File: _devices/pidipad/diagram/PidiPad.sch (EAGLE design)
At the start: 25 parts, among them IC1 CH32V006E8R6, IC2 HT7533-1, K2 MICROSD, Q1 25 MHz, X1 USB, X2 VGA, X3 AUDIO, X4 SWIO

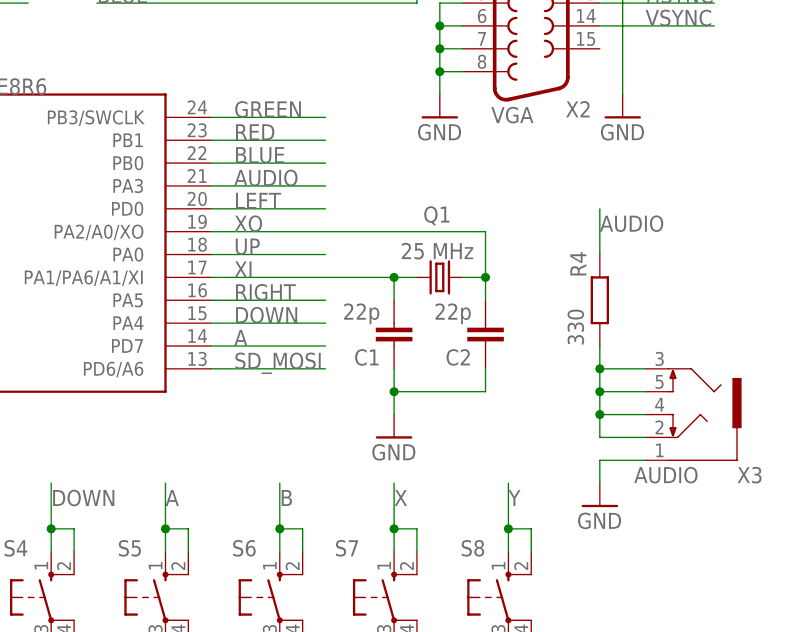
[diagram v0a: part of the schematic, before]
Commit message: init
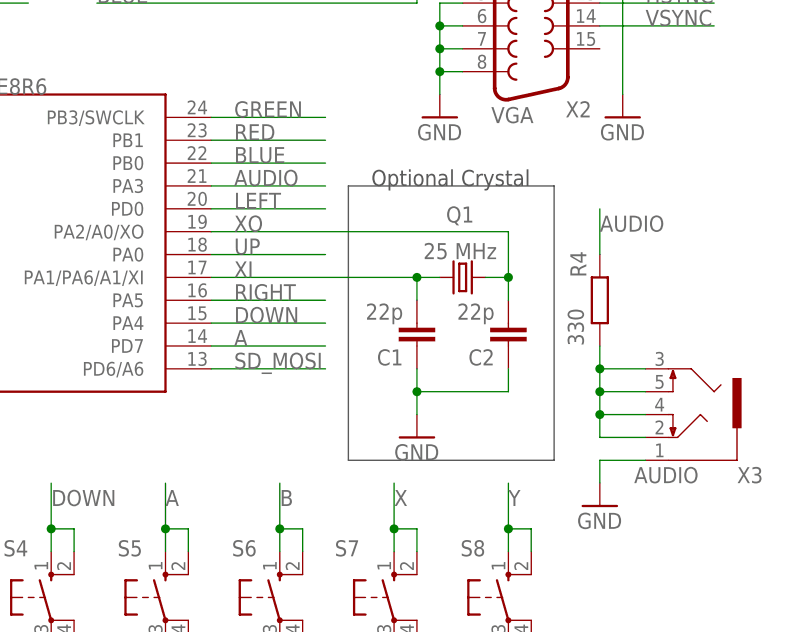
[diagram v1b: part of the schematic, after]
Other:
- note added: "Optional Crystal"
- moved on the sheet: C1, C2, Q1
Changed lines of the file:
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@@
 <setting verticaltext="up"/>
 </settings>
-<grid distance="100" unitdist="mil" unit="mil" style="lines" multiple="1" display="no" altdistance="0.01" altunitdist="inch" altunit="inch"/>
+<grid distance="0.1" unitdist="inch" unit="inch" style="lines" multiple="1" display="no" altdistance="0.01" altunitdist="inch" altunit="inch"/>
 <layers>
 <layer number="1" name="Top" color="4" fill="1" visible="no" active="no"/>
@@
 <text x="-86.36" y="0" size="1.778" layer="91">GND</text>
 <text x="-86.36" y="-2.54" size="1.778" layer="91">SWIO</text>
+<wire x1="17.78" y1="-27.94" x2="40.64" y2="-27.94" width="0.1524" layer="97"/>
+<wire x1="40.64" y1="-27.94" x2="40.64" y2="2.54" width="0.1524" layer="97"/>
+<wire x1="40.64" y1="2.54" x2="17.78" y2="2.54" width="0.1524" layer="97"/>
+<wire x1="17.78" y1="2.54" x2="17.78" y2="-27.94" width="0.1524" layer="97"/>
+<text x="20.32" y="2.54" size="1.778" layer="97">Optional Crystal</text>
 </plain>
 <instances>
@@
 <attribute name="VALUE" x="-33.02" y="12.7" size="1.778" layer="96"/>
 </instance>
-<instance part="Q1" gate="G$1" x="27.94" y="-7.62" rot="R180">
-<attribute name="NAME" x="29.21" y="0.254" size="1.778" layer="95" rot="R180"/>
-<attribute name="VALUE" x="31.75" y="-3.81" size="1.778" layer="96" rot="R180"/>
-</instance>
-<instance part="C1" gate="G$1" x="22.86" y="-15.24" rot="R180">
-<attribute name="NAME" x="21.336" y="-15.621" size="1.778" layer="95" rot="R180"/>
-<attribute name="VALUE" x="21.336" y="-10.541" size="1.778" layer="96" rot="R180"/>
-</instance>
-<instance part="C2" gate="G$1" x="33.02" y="-15.24" rot="R180">
-<attribute name="NAME" x="31.496" y="-15.621" size="1.778" layer="95" rot="R180"/>
-<attribute name="VALUE" x="31.496" y="-10.541" size="1.778" layer="96" rot="R180"/>
+<instance part="Q1" gate="G$1" x="30.48" y="-7.62" rot="R180">
+<attribute name="NAME" x="31.75" y="0.254" size="1.778" layer="95" rot="R180"/>
+<attribute name="VALUE" x="34.29" y="-3.81" size="1.778" layer="96" rot="R180"/>
+</instance>
+<instance part="C1" gate="G$1" x="25.4" y="-15.24" rot="R180">
+<attribute name="NAME" x="23.876" y="-15.621" size="1.778" layer="95" rot="R180"/>
+<attribute name="VALUE" x="23.876" y="-10.541" size="1.778" layer="96" rot="R180"/>
+</instance>
+<instance part="C2" gate="G$1" x="35.56" y="-15.24" rot="R180">
+<attribute name="NAME" x="34.036" y="-15.621" size="1.778" layer="95" rot="R180"/>
+<attribute name="VALUE" x="34.036" y="-10.541" size="1.778" layer="96" rot="R180"/>
 </instance>
 <instance part="K2" gate="G$1" x="-76.2" y="-33.02">
@@
 <attribute name="VALUE" x="-36.576" y="25.781" size="1.778" layer="96"/>
 </instance>
-<instance part="GND4" gate="1" x="22.86" y="-25.4">
-<attribute name="VALUE" x="20.32" y="-27.94" size="1.778" layer="96"/>
+<instance part="GND4" gate="1" x="25.4" y="-25.4">
+<attribute name="VALUE" x="22.86" y="-27.94" size="1.778" layer="96"/>
 </instance>
 <instance part="GND7" gate="1" x="-60.96" y="-12.7">
@@
 <segment>
 <pinref part="C1" gate="G$1" pin="1"/>
-<wire x1="22.86" y1="-17.78" x2="22.86" y2="-20.32" width="0.1524" layer="91"/>
+<wire x1="25.4" y1="-17.78" x2="25.4" y2="-20.32" width="0.1524" layer="91"/>
 <pinref part="C2" gate="G$1" pin="1"/>
-<wire x1="33.02" y1="-17.78" x2="33.02" y2="-20.32" width="0.1524" layer="91"/>
-<wire x1="33.02" y1="-20.32" x2="22.86" y2="-20.32" width="0.1524" layer="91"/>
+<wire x1="35.56" y1="-17.78" x2="35.56" y2="-20.32" width="0.1524" layer="91"/>
+<wire x1="35.56" y1="-20.32" x2="25.4" y2="-20.32" width="0.1524" layer="91"/>
 <pinref part="GND4" gate="1" pin="GND"/>
-<wire x1="22.86" y1="-22.86" x2="22.86" y2="-20.32" width="0.1524" layer="91"/>
-<junction x="22.86" y="-20.32"/>
+<wire x1="25.4" y1="-22.86" x2="25.4" y2="-20.32" width="0.1524" layer="91"/>
+<junction x="25.4" y="-20.32"/>
 </segment>
 <segment>
@@
 <pinref part="IC1" gate="G$1" pin="PA1/PA6/A1/XI"/>
 <pinref part="Q1" gate="G$1" pin="2"/>
-<wire x1="2.54" y1="-7.62" x2="22.86" y2="-7.62" width="0.1524" layer="91"/>
+<wire x1="2.54" y1="-7.62" x2="25.4" y2="-7.62" width="0.1524" layer="91"/>
 <pinref part="C1" gate="G$1" pin="2"/>
-<wire x1="22.86" y1="-7.62" x2="25.4" y2="-7.62" width="0.1524" layer="91"/>
-<wire x1="22.86" y1="-10.16" x2="22.86" y2="-7.62" width="0.1524" layer="91"/>
-<junction x="22.86" y="-7.62"/>
+<wire x1="25.4" y1="-7.62" x2="27.94" y2="-7.62" width="0.1524" layer="91"/>
+<wire x1="25.4" y1="-10.16" x2="25.4" y2="-7.62" width="0.1524" layer="91"/>
+<junction x="25.4" y="-7.62"/>
 <label x="5.08" y="-7.62" size="1.778" layer="95"/>
 </segment>
@@
 <segment>
 <pinref part="C2" gate="G$1" pin="2"/>
-<wire x1="33.02" y1="-10.16" x2="33.02" y2="-7.62" width="0.1524" layer="91"/>
+<wire x1="35.56" y1="-10.16" x2="35.56" y2="-7.62" width="0.1524" layer="91"/>
 <pinref part="Q1" gate="G$1" pin="1"/>
-<wire x1="33.02" y1="-7.62" x2="30.48" y2="-7.62" width="0.1524" layer="91"/>
+<wire x1="35.56" y1="-7.62" x2="33.02" y2="-7.62" width="0.1524" layer="91"/>
 <pinref part="IC1" gate="G$1" pin="PA2/A0/XO"/>
-<wire x1="2.54" y1="-2.54" x2="33.02" y2="-2.54" width="0.1524" layer="91"/>
-<wire x1="33.02" y1="-2.54" x2="33.02" y2="-7.62" width="0.1524" layer="91"/>
-<junction x="33.02" y="-7.62"/>
+<wire x1="2.54" y1="-2.54" x2="35.56" y2="-2.54" width="0.1524" layer="91"/>
+<wire x1="35.56" y1="-2.54" x2="35.56" y2="-7.62" width="0.1524" layer="91"/>
+<junction x="35.56" y="-7.62"/>
 <label x="5.08" y="-2.54" size="1.778" layer="95"/>
 </segment>
